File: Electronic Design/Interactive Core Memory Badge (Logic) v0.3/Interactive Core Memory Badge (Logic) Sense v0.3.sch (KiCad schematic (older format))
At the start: 21 parts, among them U3 LM393, U4 74HC02

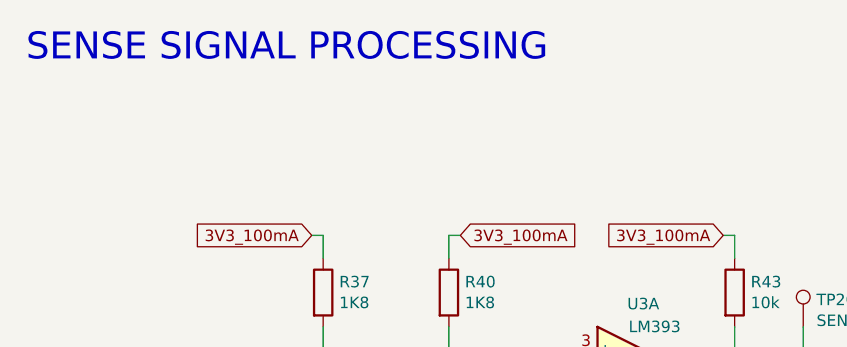
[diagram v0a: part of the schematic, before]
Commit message: Schematic refinement
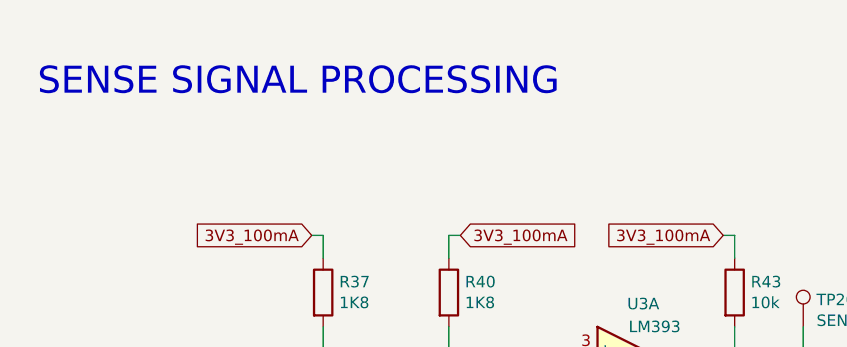
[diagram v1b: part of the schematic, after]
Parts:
- U4: footprint (none) -> Package_SO:SOIC-14_3.9x8.7mm_P1.27mm
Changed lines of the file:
@@
 $Descr A4 11693 8268
 encoding utf-8
-Sheet 5 6
+Sheet 3 5
 Title "Core 64 - Sense"
 Date "2020-03-15"
@@
 Comment4 ""
 $EndDescr
-Text Notes 550  700  0    118  ~ 0
+Text Notes 600  850  0    118  ~ 0
 SENSE SIGNAL PROCESSING
 $Comp
@@
 F 0 "U4" H 5100 2929 50  0000 C CNN
 F 1 "74HC02" H 5100 2836 50  0000 C CNN
-F 2 "" H 5100 2600 50  0001 C CNN
+F 2 "Package_SO:SOIC-14_3.9x8.7mm_P1.27mm" H 5100 2600 50  0001 C CNN
 F 3 "http://www.ti.com/lit/gpn/sn74hc02" H 5100 2600 50  0001 C CNN
 	1    5100 2600
@@
 F 0 "U4" H 5800 2929 50  0000 C CNN
 F 1 "74HC02" H 5800 2836 50  0000 C CNN
-F 2 "" H 5800 2600 50  0001 C CNN
+F 2 "Package_SO:SOIC-14_3.9x8.7mm_P1.27mm" H 5800 2600 50  0001 C CNN
 F 3 "http://www.ti.com/lit/gpn/sn74hc02" H 5800 2600 50  0001 C CNN
 	2    5800 2600
@@
 F 0 "U4" H 6500 2050 50  0000 C CNN
 F 1 "74HC02" H 6550 1950 50  0000 C CNN
-F 2 "" H 6600 1750 50  0001 C CNN
+F 2 "Package_SO:SOIC-14_3.9x8.7mm_P1.27mm" H 6600 1750 50  0001 C CNN
 F 3 "http://www.ti.com/lit/gpn/sn74hc02" H 6600 1750 50  0001 C CNN
 	3    6600 1750
@@
 F 0 "U4" H 6500 2800 50  0000 C CNN
 F 1 "74HC02" H 6550 2700 50  0000 C CNN
-F 2 "" H 6600 2500 50  0001 C CNN
+F 2 "Package_SO:SOIC-14_3.9x8.7mm_P1.27mm" H 6600 2500 50  0001 C CNN
 F 3 "http://www.ti.com/lit/gpn/sn74hc02" H 6600 2500 50  0001 C CNN
 	4    6600 2500
@@
 F 0 "U4" H 5380 3697 50  0000 L CNN
 F 1 "74HC02" H 5380 3604 50  0000 L CNN
-F 2 "" H 5150 3650 50  0001 C CNN
+F 2 "Package_SO:SOIC-14_3.9x8.7mm_P1.27mm" H 5150 3650 50  0001 C CNN
 F 3 "http://www.ti.com/lit/gpn/sn74hc02" H 5150 3650 50  0001 C CNN
 	5    5150 3650
